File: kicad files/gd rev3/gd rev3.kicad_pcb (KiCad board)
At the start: 4 copper layers, 286 parts, among them J1 XY, J10 Apple_II_Slot, J11 Game Port, J12 Right Angle, J13 SWD, J14 USB_A, J15 Rev2 Header, J16 RP2040 Header, J17 VGA_Micro, J18 vga_SWD, J19 SPKR, J2 DB19_4, J20 Ears, J21 KBD Serial, J22 L77HDE15SD1CH4F, J23 Game-DB VERIFY FOOTPRINT, J3 DB19_16, J4 EN, J5 DSUB19, J6 FDC Hdr, J7 EN, J8 EN, J9 IO-Xtra, Q1 BC817, Q2 BC817, Q3 BC817, Q4 BC817, Q5 BC817, Q6 BC817, Q7 BC817, Q8 BC817, Q9 BC817, SW1 MEGA RESET, SW2 DEV, SW3 IOSEL, SW4 KBD RESET, SW5 KBD Boot Sel, SW6 VGA Boot Sel, SW7 VGA RESET, U1 Apple_MEGA_II, U10 DRAM64KX4, U11 IWM, U12 Slotmaker, U13 74HCT245, U14 RP2040, U15 MIC5504-3.3YM5, U16 74HC245, U17 W25Q128JVS, U18 HCT251, U19 W25Q128JVS, U2 w65c02s, U20 NE556, U21 NE556, U22 74HCT245, U23 RP2040, U24 74LVC2G04, U26 MCP4541T, U27 LM4875, U28 SN74LVC573ANS, U29 74LVC2G04, U3 74LVC1G02, U30 74LVC2G04, U32 LM7905_TO220, U35 74LVC2G04, U4 74HCT245, U5 74HCT245, U6 AT28C256-PLCC, U7 DRAM64KX4, U8 DRAM64KX4, U9 DRAM64KX4, X1 14.31818MHz, Y1 ECS-120-18-33-JEM-TR, Y2 ECS-120-18-33-JEM-TR

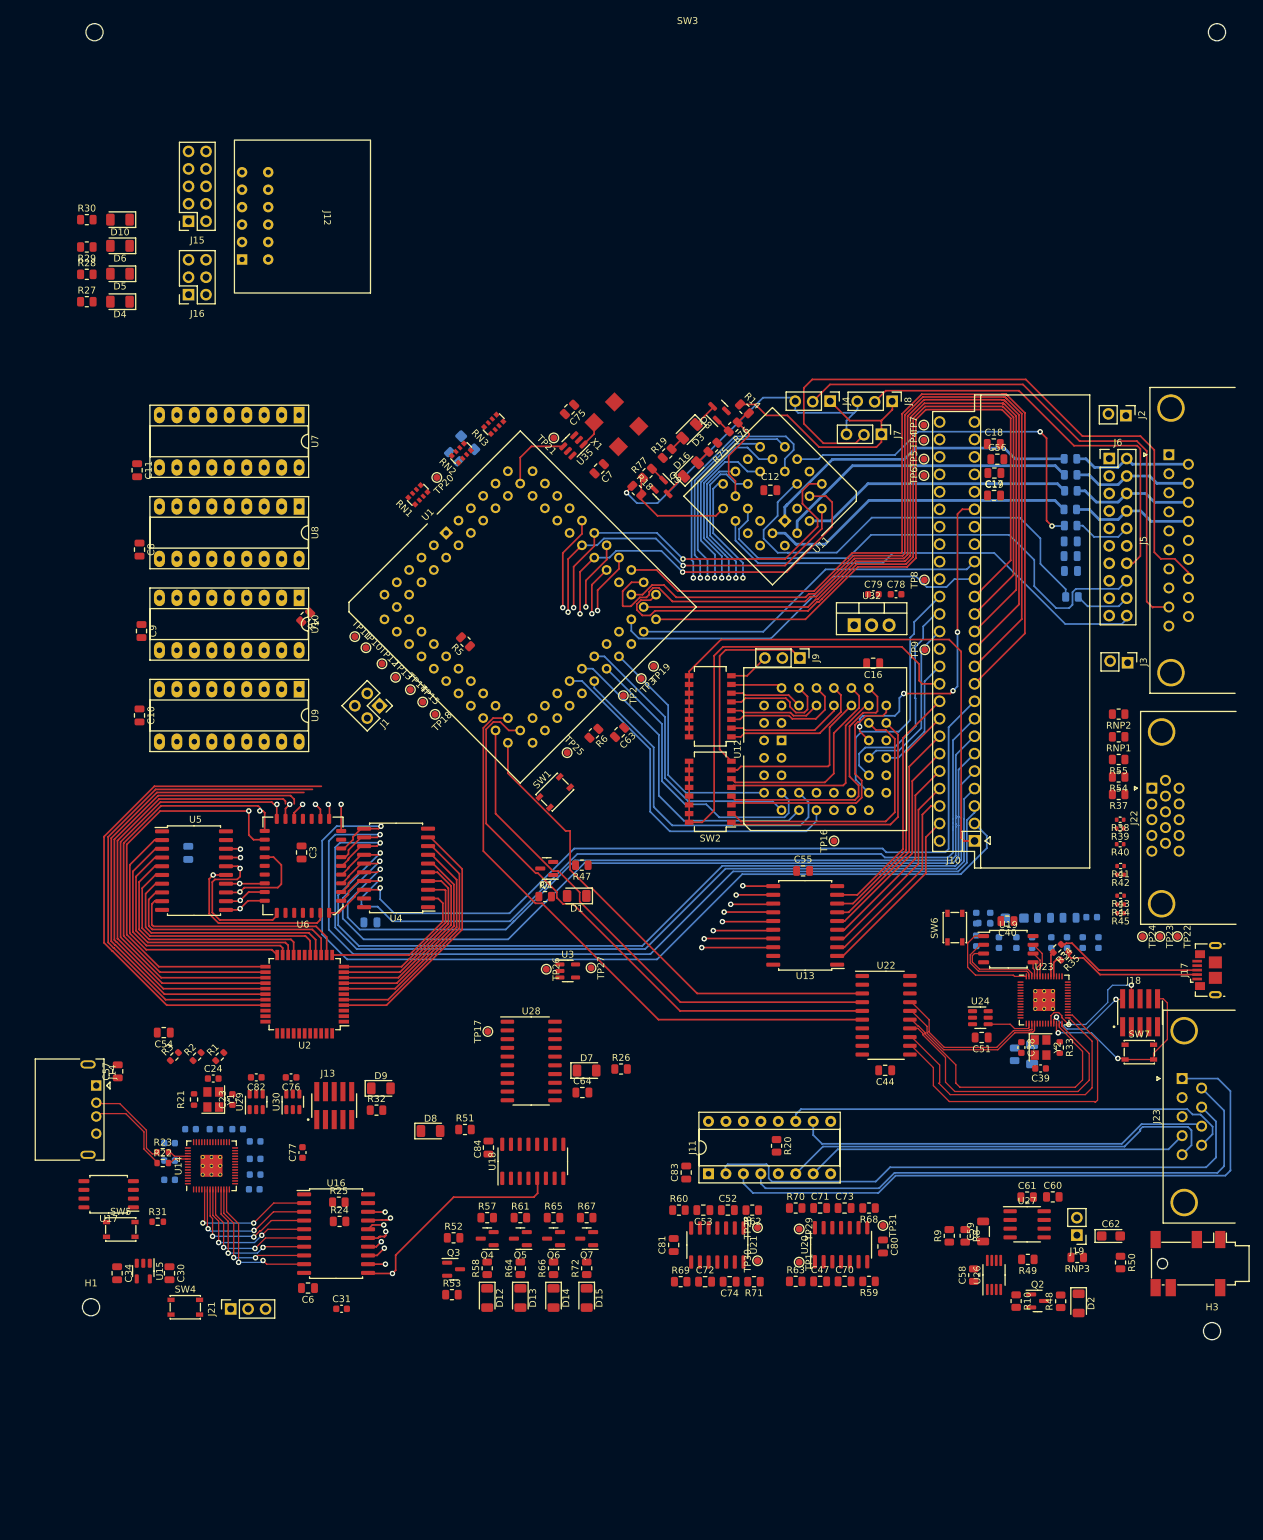
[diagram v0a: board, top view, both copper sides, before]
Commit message: re-arranged everything... what have I done?!
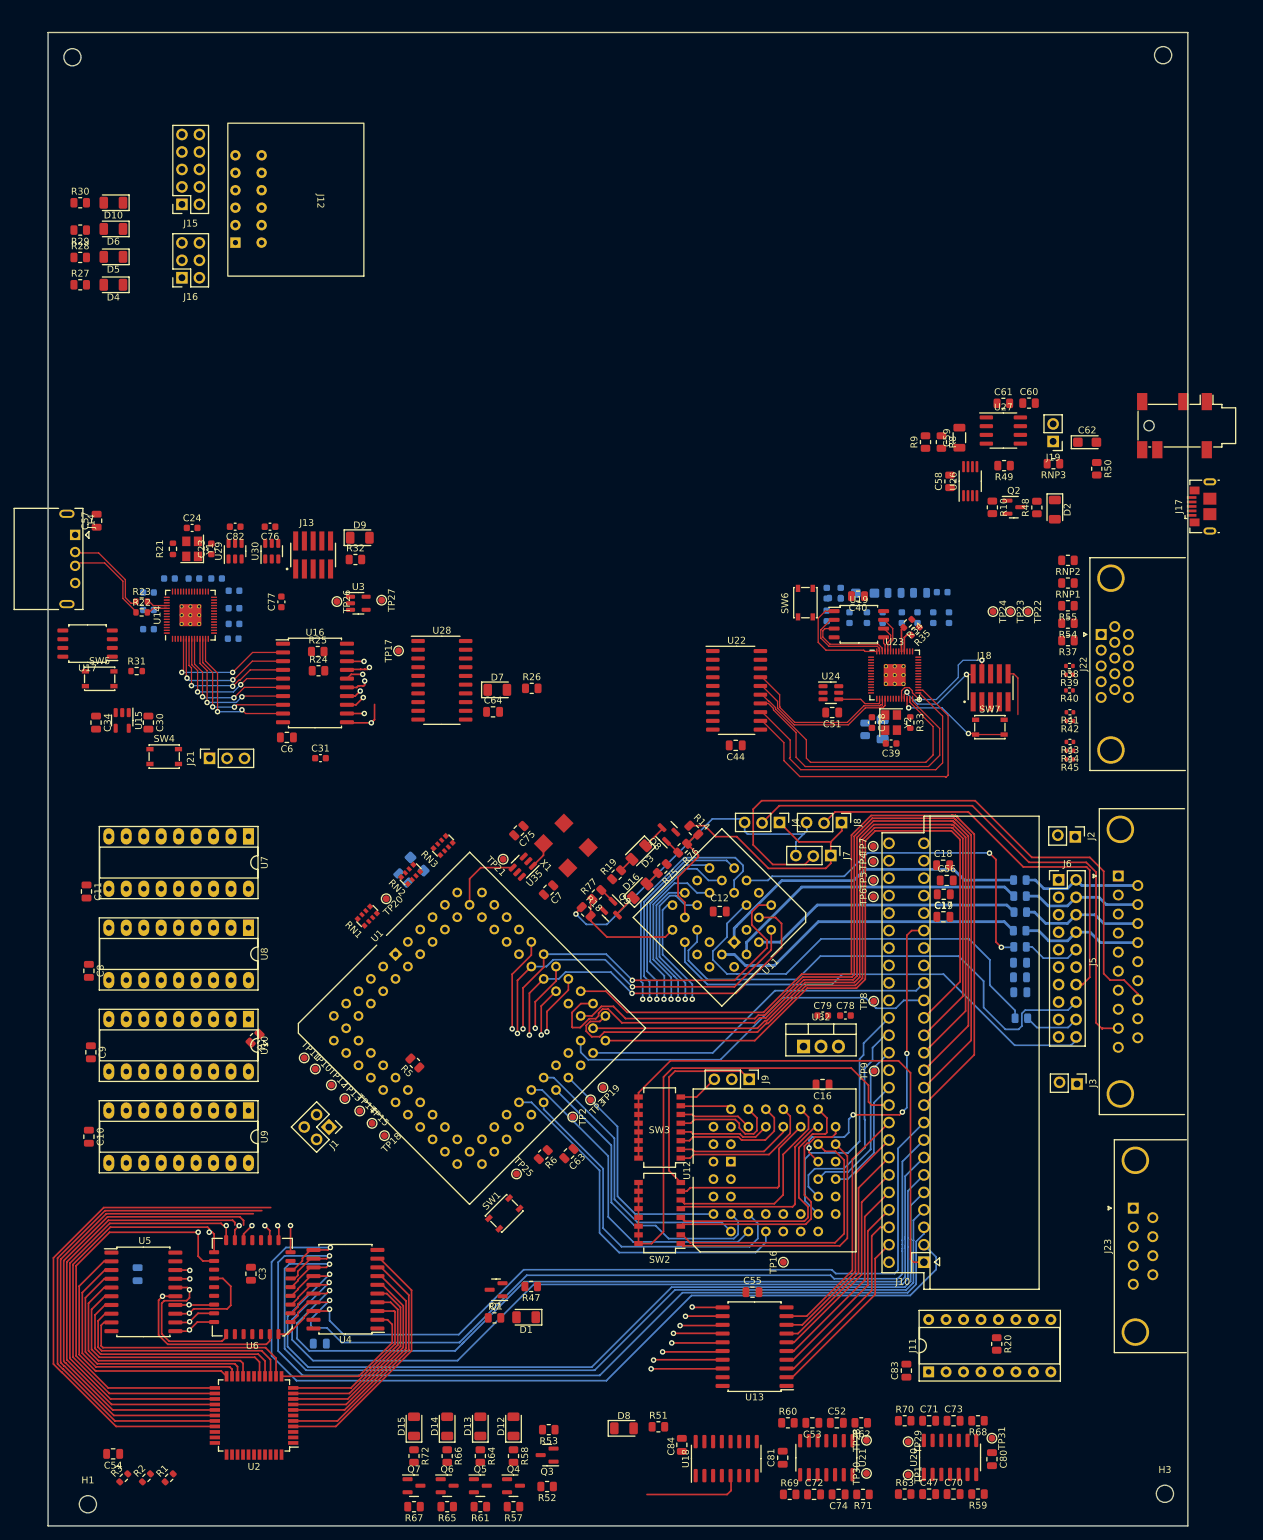
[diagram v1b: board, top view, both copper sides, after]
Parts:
- moved J20 121.9 mm to (224.7, 86.4)
- moved R10 115.6 mm to (198.2, 98.2)
- moved U26 115.6 mm to (195.0, 94.4)
- moved C58 115.6 mm to (192.0, 94.5)
- moved C59 115.6 mm to (193.4, 88.1)
- moved C60 115.6 mm to (203.5, 83.1)
- moved D2 115.6 mm to (207.3, 98.6)
- moved J19 115.6 mm to (207.0, 88.6)
- moved R48 115.6 mm to (204.7, 98.3)
- moved R49 115.6 mm to (199.9, 92.2)
- moved R50 115.6 mm to (213.4, 92.6)
- moved R8 115.6 mm to (190.8, 88.7)
- moved R9 115.6 mm to (188.5, 88.7)
- moved U27 115.6 mm to (199.8, 87.1)
- moved C61 115.6 mm to (199.8, 83.1)
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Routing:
- net /game_port/SW1_CAPL: track 93.5 -> 0.00 mm
- net /IWM/MD7: track 420.4 -> 330.4 mm
- net /mega-6502/RGB4: track 87.4 -> 0.00 mm
- net /mega-6502/RGB1: track 86.1 -> 0.00 mm
- net /game_port/SW0_OAPL: track 84.2 -> 0.00 mm
- net /game_port/SW2: track 83.2 -> 0.00 mm
- net /mega-6502/RGB8: track 77.6 -> 0.00 mm
- net /mega-6502/RGB2: track 72.6 -> 0.00 mm
- net /IWM/MD6: track 396.3 -> 327.0 mm
- net /IWM/MD5: track 384.6 -> 316.6 mm
- net /IWM/MD4: track 393.3 -> 325.9 mm
- net /game_port/PDL3: track 66.4 -> 0.00 mm
- net /IWM/MD3: track 395.4 -> 329.2 mm
- net /IWM/MD2: track 393.2 -> 328.1 mm
- net /game_port/PDL0: track 64.9 -> 0.00 mm
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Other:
- board outline added: 165.9 x 217.3 mm
